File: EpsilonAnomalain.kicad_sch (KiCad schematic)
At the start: 96 parts, among them J1 I2C, J2 ServoA, J3 ServoB, J4 ServoC, J5 ServoD, J6 USB_C, J7 Power, J8 UART, Q1 BC817-40, SW1 ON, SW2 ON, SW3 ON, U1 ESP32-S3FN8, U10 USBLC6-2SC6, U2 ICM-42688-P, U3 BMP388, U4 AHT20, U5 W25N01GVZEIG, U6 SS206SURWA/S530-A3/S290, U7 74HC595, U8 TPS61088, U9 AP2112K-3.3, Y1 40 MHz

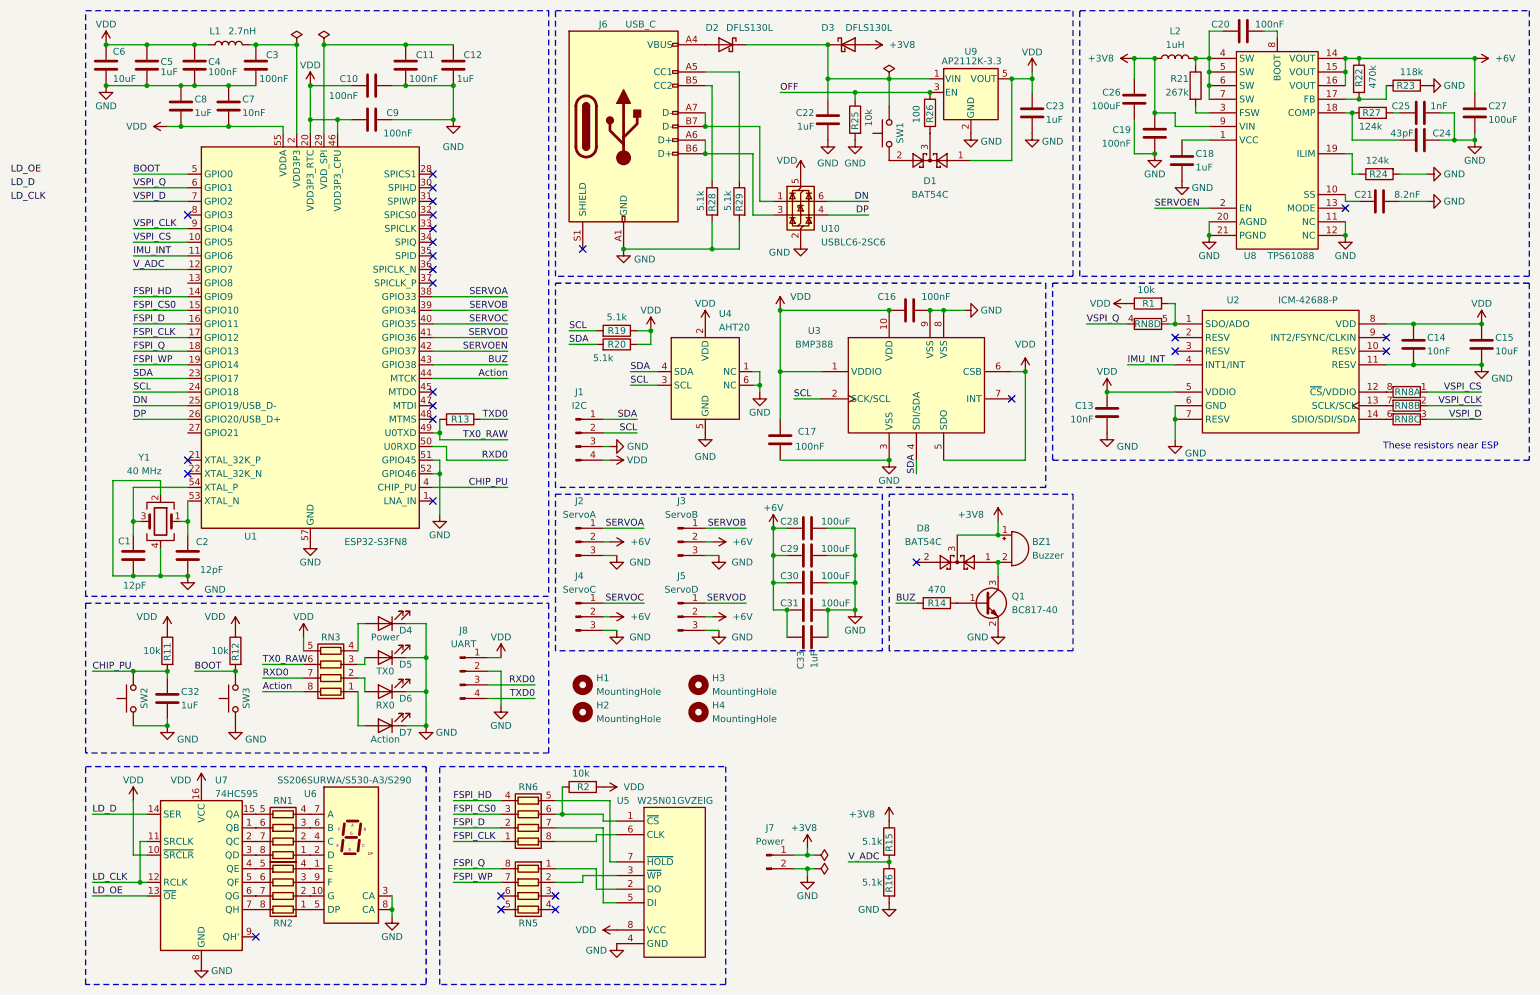
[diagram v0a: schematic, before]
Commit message: v2.20
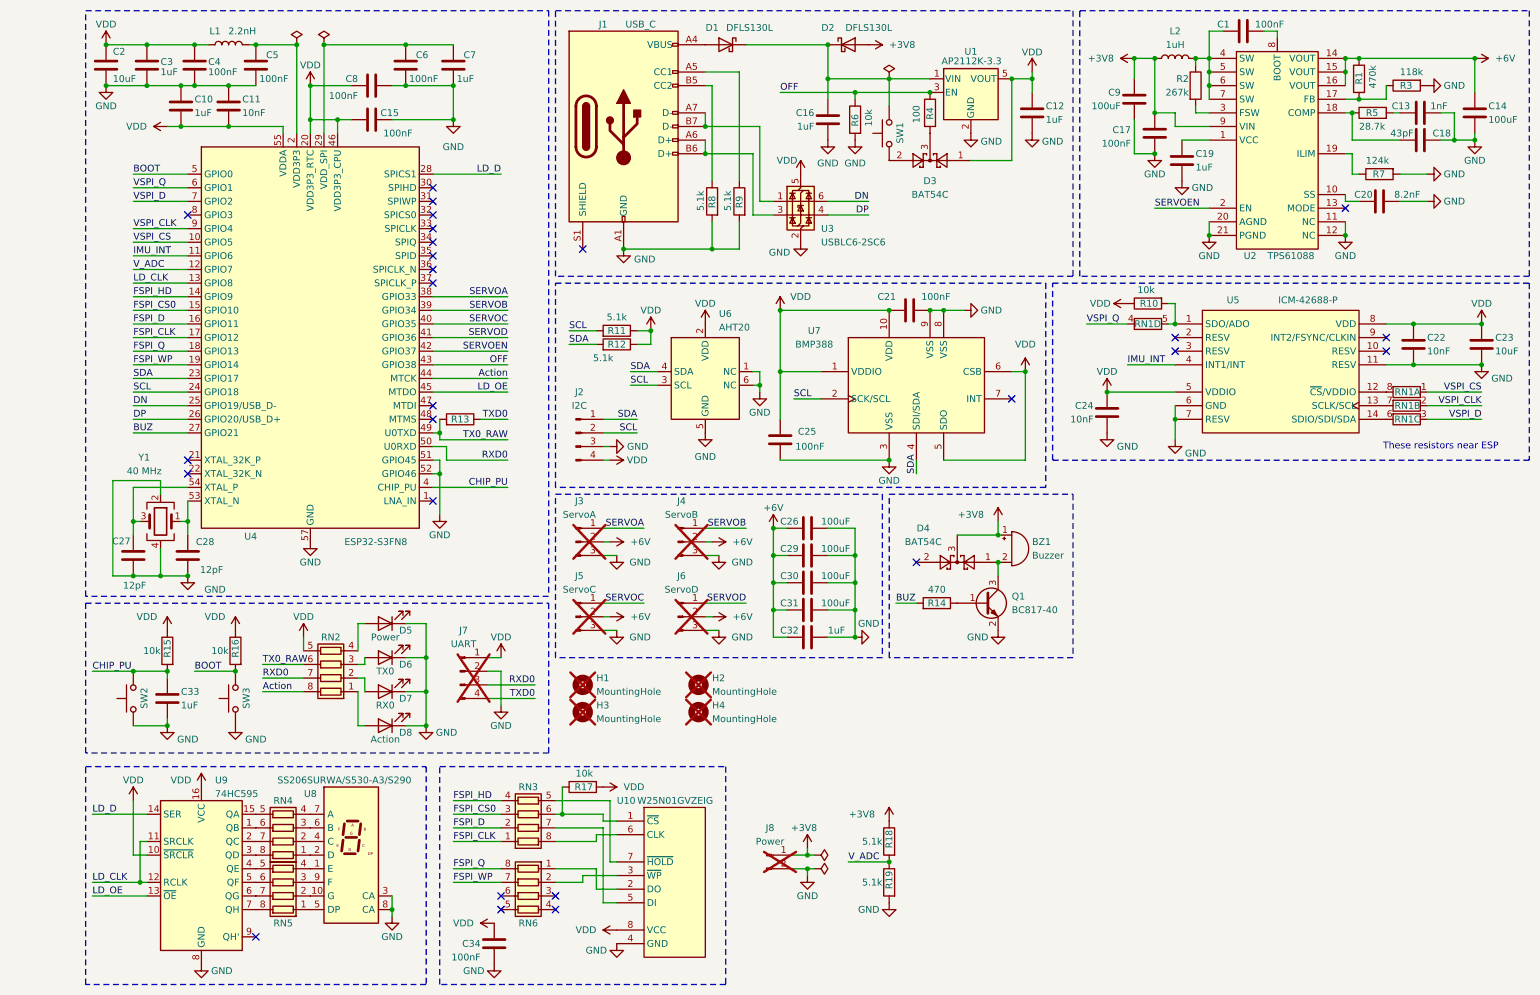
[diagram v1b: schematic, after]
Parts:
- added C34: 100nF, Capacitor_SMD:C_0402_1005Metric, symbol Device:C
- H1, H4: now not fitted
- H2: renamed from H3; now not fitted
- H3: renamed from H2; now not fitted
- J3: renamed from J2; now not fitted
- J4: renamed from J3; now not fitted
- J5: renamed from J4; now not fitted
- J6: renamed from J5; now not fitted
- J7: renamed from J8; now not fitted
- J8: renamed from J7; now not fitted
- L1: value 2.7nH -> 2.2nH
- R5: renamed from R27; value 124k -> 28.7k
- RN1: renamed from RN8; value R_Pack04_Split -> 47
- renumbered C20 to C1, C8 to C10, C7 to C11, C23 to C12, C25 to C13, C27 to C14, C9 to C15, C22 to C16, C19 to C17, C24 to C18, C18 to C19, C6 to C2, C21 to C20, C16 to C21, C14 to C22, C15 to C23, C13 to C24, C17 to C25, C28 to C26, C1 to C27, C2 to C28, C5 to C3, C33 to C32, C32 to C33, C3 to C5, C11 to C6, C12 to C7, C10 to C8, C26 to C9, D2 to D1, D3 to D2, D1 to D3, D8 to D4, D4 to D5, D5 to D6, D6 to D7, D7 to D8, J6 to J1, J1 to J2, R22 to R1, R1 to R10, R19 to R11, R20 to R12, R11 to R15, R12 to R16, R2 to R17, R15 to R18, R16 to R19, R21 to R2, R23 to R3, R26 to R4, R25 to R6, R24 to R7, R28 to R8, R29 to R9, RN3 to RN2, RN6 to RN3, RN1 to RN4, RN2 to RN5, RN5 to RN6, U9 to U1, U5 to U10, U8 to U2, U10 to U3, U1 to U4, U2 to U5, U4 to U6, U3 to U7, U6 to U8, U7 to U9
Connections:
- net BUZ: now also U4.27 (GPIO21); no longer U4.43 (GPIO38)
- net GND: now also C34.2
- net LD_CLK: now also U4.13 (GPIO8)
- net LD_D: now also U4.28 (SPICS1)
- net LD_OE: now also U4.45 (MTDO)
- net OFF: now also U4.43 (GPIO38)
- net VDD: now also C34.1
- no-connect marks 29 -> 27

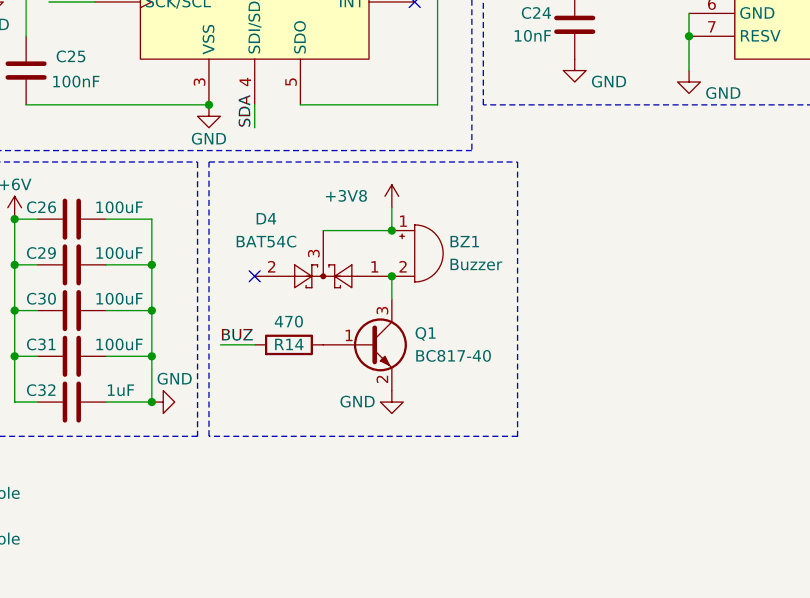
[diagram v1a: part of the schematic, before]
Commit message: v2.22
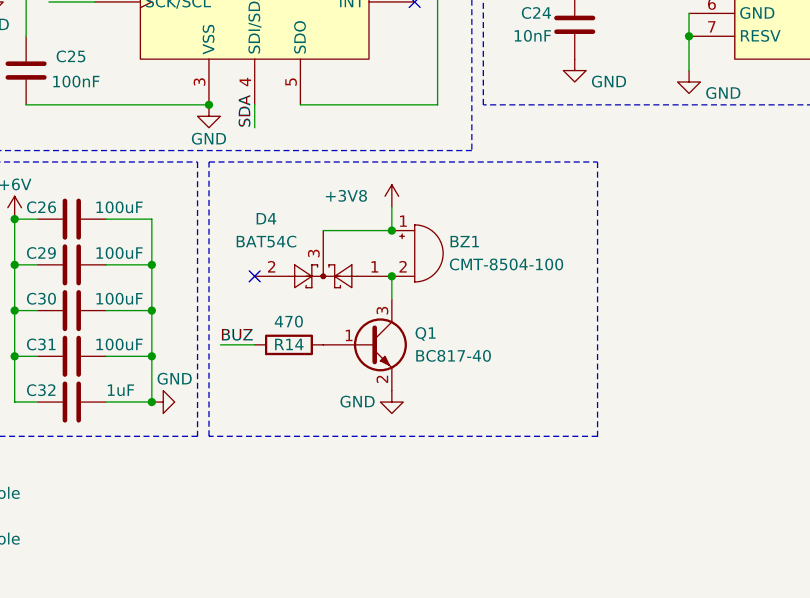
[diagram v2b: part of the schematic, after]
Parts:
- BZ1: value Buzzer -> CMT-8504-100; Mfr.Part (none) -> CMT-8504-100
- J1: Mfr.Part (none) -> TYPE C-DB-116PWB
- J2: Mfr.Part (none) -> A1257WR-S-4P
- L2: Mfr.Part (none) -> APH0630T1R0M
- SW1, SW2, SW3: value ON -> TS-1187A-B-A-B; Mfr.Part (none) -> TS-1187A-B-A-B
- U1: Mfr.Part (none) -> AP2112K-3.3
- U10: Mfr.Part (none) -> W25N01GVZEIG
- U2: Mfr.Part (none) -> TPS61088
- U3: Mfr.Part (none) -> USBLC6-2SC6
- U4: Mfr.Part (none) -> ESP32-S3FN8
- U5: Mfr.Part (none) -> ICM-42688-P
- U6: Mfr.Part (none) -> AHT20
- U7: footprint CustomPackage:BMP388 -> CustomPackage:BMP388_v2; Mfr.Part (none) -> BMP388
- U8: Mfr.Part (none) -> SS206SURWA/S530-A3/S290

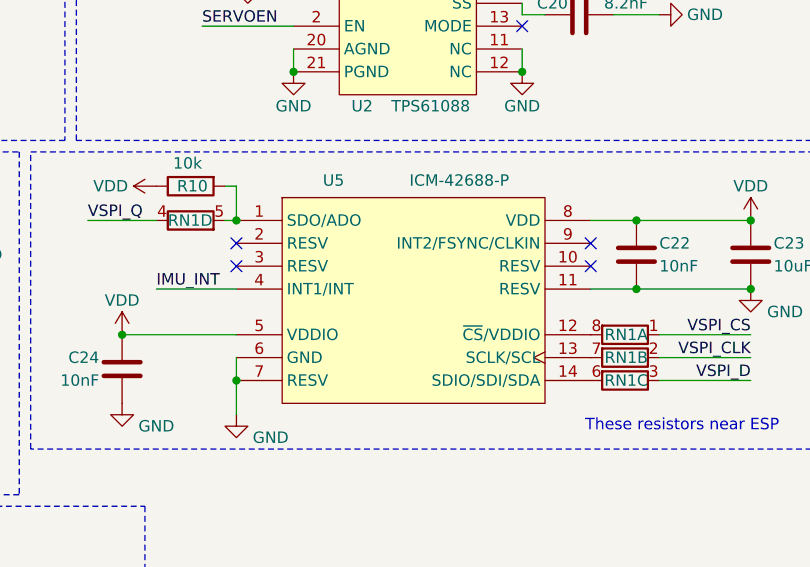
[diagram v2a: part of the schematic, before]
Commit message: update
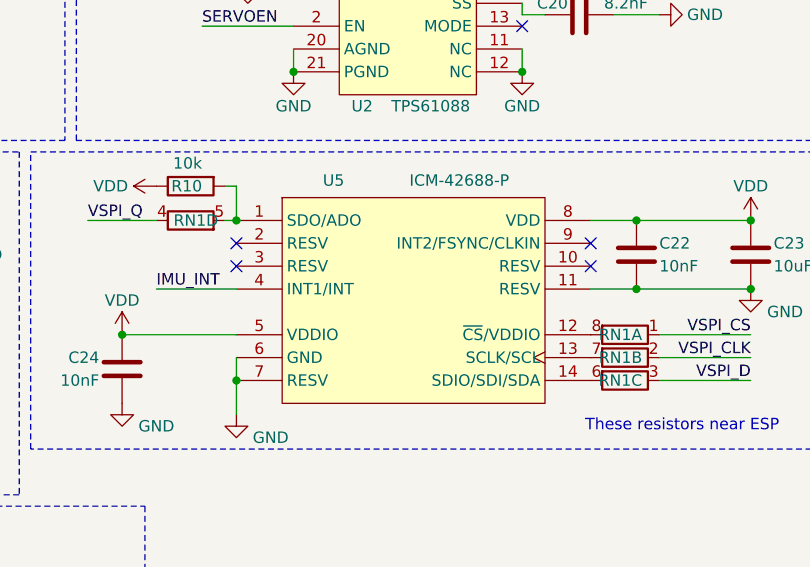
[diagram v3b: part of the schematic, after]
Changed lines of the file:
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@@
 		(dnp no)
 		(property "Reference" "RN1"
-			(at 209.55 72.39 90)
+			(at 210.185 72.39 90)
 			(effects
 				(font
@@
 		(dnp no)
 		(property "Reference" "R10"
-			(at 213.995 68.58 90)
+			(at 213.36 68.58 90)
 			(effects
 				(font
@@
 		(dnp no)
 		(property "Reference" "RN1"
-			(at 262.89 87.63 90)
+			(at 262.255 87.63 90)
 			(effects
 				(font
@@
 		(dnp no)
 		(property "Reference" "RN1"
-			(at 262.89 90.17 90)
+			(at 262.255 90.17 90)
 			(effects
 				(font
@@
 		(dnp no)
 		(property "Reference" "RN1"
-			(at 262.89 85.09 90)
+			(at 262.255 85.09 90)
 			(effects
 				(font
